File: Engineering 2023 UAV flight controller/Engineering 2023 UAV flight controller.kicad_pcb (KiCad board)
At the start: 4 copper layers, 70 x 120 mm, 86 parts, among them J1 Micro_SD_Card, J2 ESC speed control, J3 USB_C_Receptacle_USB2.0, J4 Conn_Coaxial, J5 external power rail, J6 Board GPIO and the Lora DIO, J7 external ground rail, M1 Aileron Left, M2 Aileron Right, M3 Elevator Left, M4 Elevator Right, SW1 SW_SPDT, SW2 4FSH922, SW3 SW_Push, U1 W25Q128JVS, U2 NCP1117-3.3_TO252, U3 LM350_TO220, U4 RP2040, U5 LPS25HB, U6 MPU-6050, U7 MMC5983MA, U8 E28-2G4M27S, U9 NEO-M8N, Y1 ABLS-12.000MHZ-B4-T

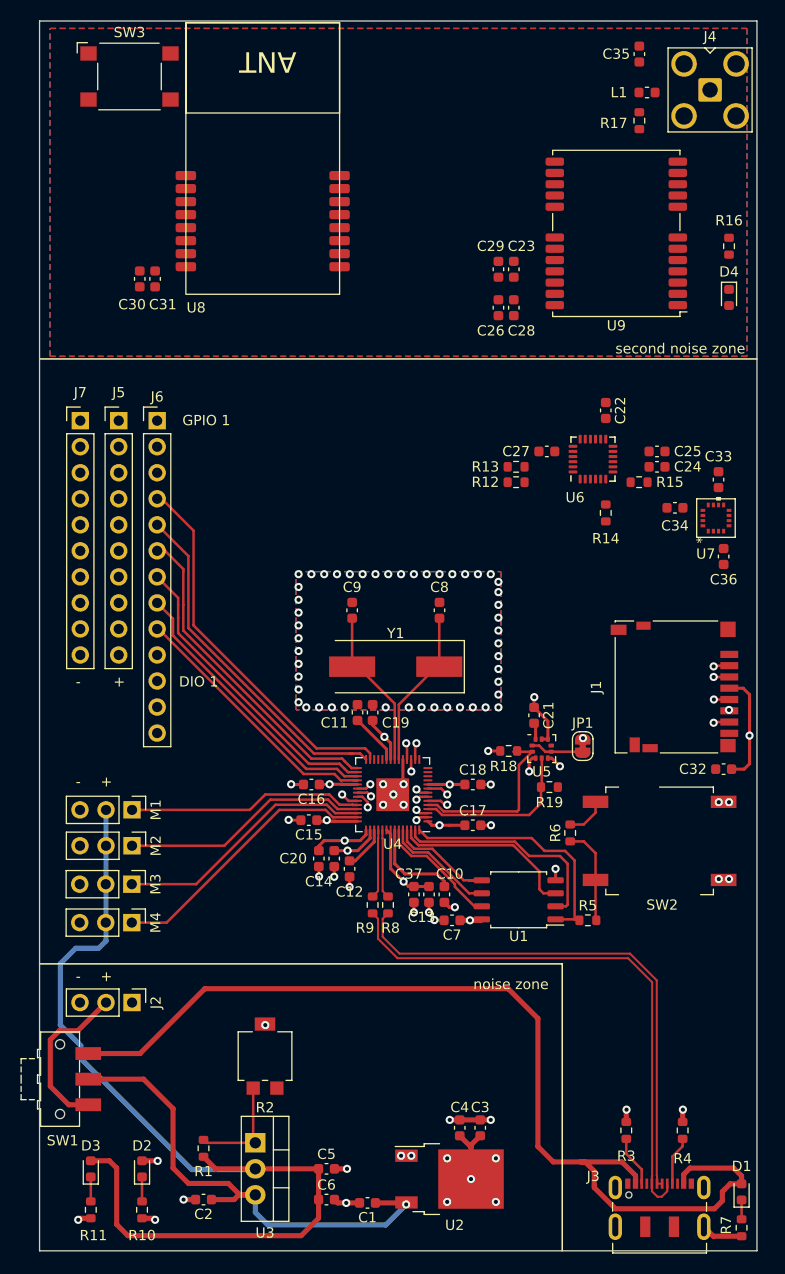
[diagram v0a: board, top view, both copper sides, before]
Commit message: pcb revision one completed, the png's are for the reddit gods to review.
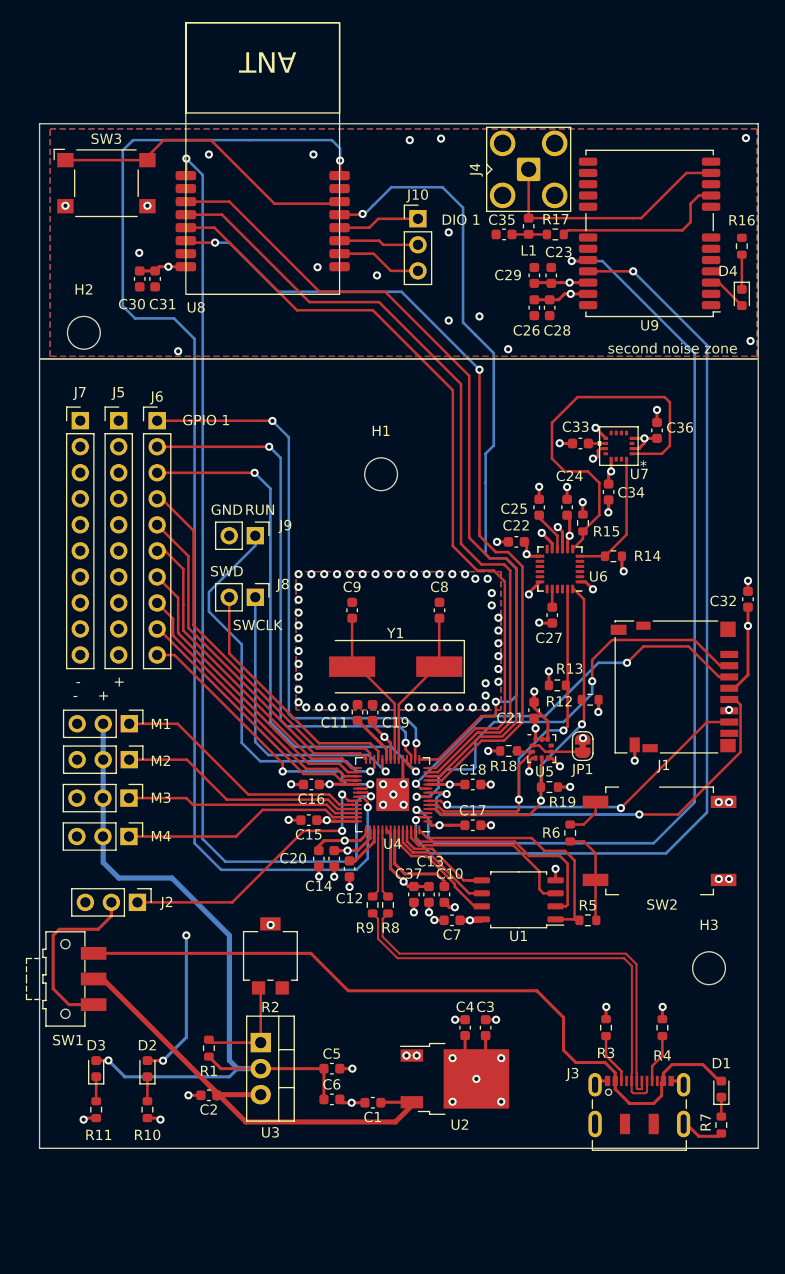
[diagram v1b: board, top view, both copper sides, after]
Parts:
- added H1: MountingHole, MountingHole:MountingHole_3.2mm_M3, F.Cu at (148.8, 76.0)
- added H2: MountingHole, MountingHole:MountingHole_3.2mm_M3, F.Cu at (119.8, 62.2)
- added H3: MountingHole, MountingHole:MountingHole_3.2mm_M3, F.Cu at (180.8, 124.2)
- added J10: DIO, Connector_PinHeader_2.54mm:PinHeader_1x03_P2.54mm_Vertical, F.Cu at (152.4, 51.1)
- added J8: Serial wire debug, Connector_PinHeader_2.54mm:PinHeader_1x02_P2.54mm_Vertical, F.Cu at (136.5, 88.0)
- added J9: reset short?, Connector_PinHeader_2.54mm:PinHeader_1x02_P2.54mm_Vertical, F.Cu at (136.5, 82.0)
- J6: value Board GPIO and the Lora DIO -> GPIO; footprint Connector_PinHeader_2.54mm:PinHeader_1x13_P2.54mm_Vertical -> Connector_PinHeader_2.54mm:PinHeader_1x10_P2.54mm_Vertical
- moved R12 22.4 mm to (169.2, 98.0), turned to 0 degrees
- moved C35 22.0 mm to (160.8, 52.6), turned to 180 degrees
- moved R13 21.7 mm to (166.0, 96.6)
- moved J4 19.3 mm to (163.2, 46.2), turned to 0 degrees
- moved L1 17.4 mm to (163.2, 51.8), turned to 90 degrees
- moved C32 16.7 mm to (184.6, 88.2), turned to 90 degrees
- moved C27 16.0 mm to (165.5, 89.8), turned to 90 degrees
- moved C22 15.5 mm to (162.0, 82.6), turned to 0 degrees
- moved C33 13.9 mm to (168.2, 73.0), turned to 0 degrees
- moved C36 13.9 mm to (175.7, 71.7), turned to -90 degrees
- moved R17 13.8 mm to (165.8, 52.6), turned to 180 degrees
- moved C25 12.7 mm to (164.2, 79.2), turned to -90 degrees
- moved U7 11.8 mm to (172.0, 73.2), turned to 180 degrees
- moved U6 11.2 mm to (166.2, 85.2), turned to 180 degrees
- moved SW3 10.7 mm to (122.0, 47.6)
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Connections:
- C25 pad 2: /IMU_decouple_cap -> /IMU_REGOUT
- C27 pad 2: /IMU_decouple_cap -> /IMU_CPOUT
- U6 pad 10: /IMU_decouple_cap -> /IMU_REGOUT
- U6 pad 20: /IMU_decouple_cap -> /IMU_CPOUT
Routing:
- net /LORA_TX_EN: track 1.73 -> 122.5 mm, vias 1 -> 2
- net /NEO_RXD: track 1.23 -> 94.0 mm, vias 1 -> 2
- net /NEO_TXD: track 1.25 -> 93.6 mm, vias 1 -> 2
- net /LORA_RX_EN: track 1.47 -> 93.5 mm, vias 1 -> 2
- net /LORA_MISO: track 0.00 -> 82.3 mm, vias 0 -> 2
- net /LORA_~{SS}: track 0.00 -> 82.1 mm
- net /LORA SCK: track 0.00 -> 80.0 mm
- net /LORA_BUSY: track 0.00 -> 78.1 mm, vias 0 -> 2
- net /LORA_MOSI: track 0.00 -> 77.4 mm
- net /External_pin_1: track 1.63 -> 56.6 mm, vias 1 -> 2
- net /External_pin_2: track 1.18 -> 53.6 mm, vias 1 -> 2
- net /External_pin_3: track 1.62 -> 52.3 mm, vias 1 -> 2
- net /3.3v rail: track 93.9 -> 135.7 mm, vias 20 -> 34
- net /microSD_CS: track 2.79 -> 43.1 mm
- net /microSD_CLK: track 2.76 -> 42.5 mm
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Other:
- board size 70 x 120 mm -> 70.1 x 100 mm
- board text added: "GND"
- board text added: "RUN"
- board text added: "SWCLK"
- board text added: "SWD"
- board text removed: "no reason to put anything here"
- board text removed: "noise zone"
